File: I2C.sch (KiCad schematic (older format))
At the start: 10 parts

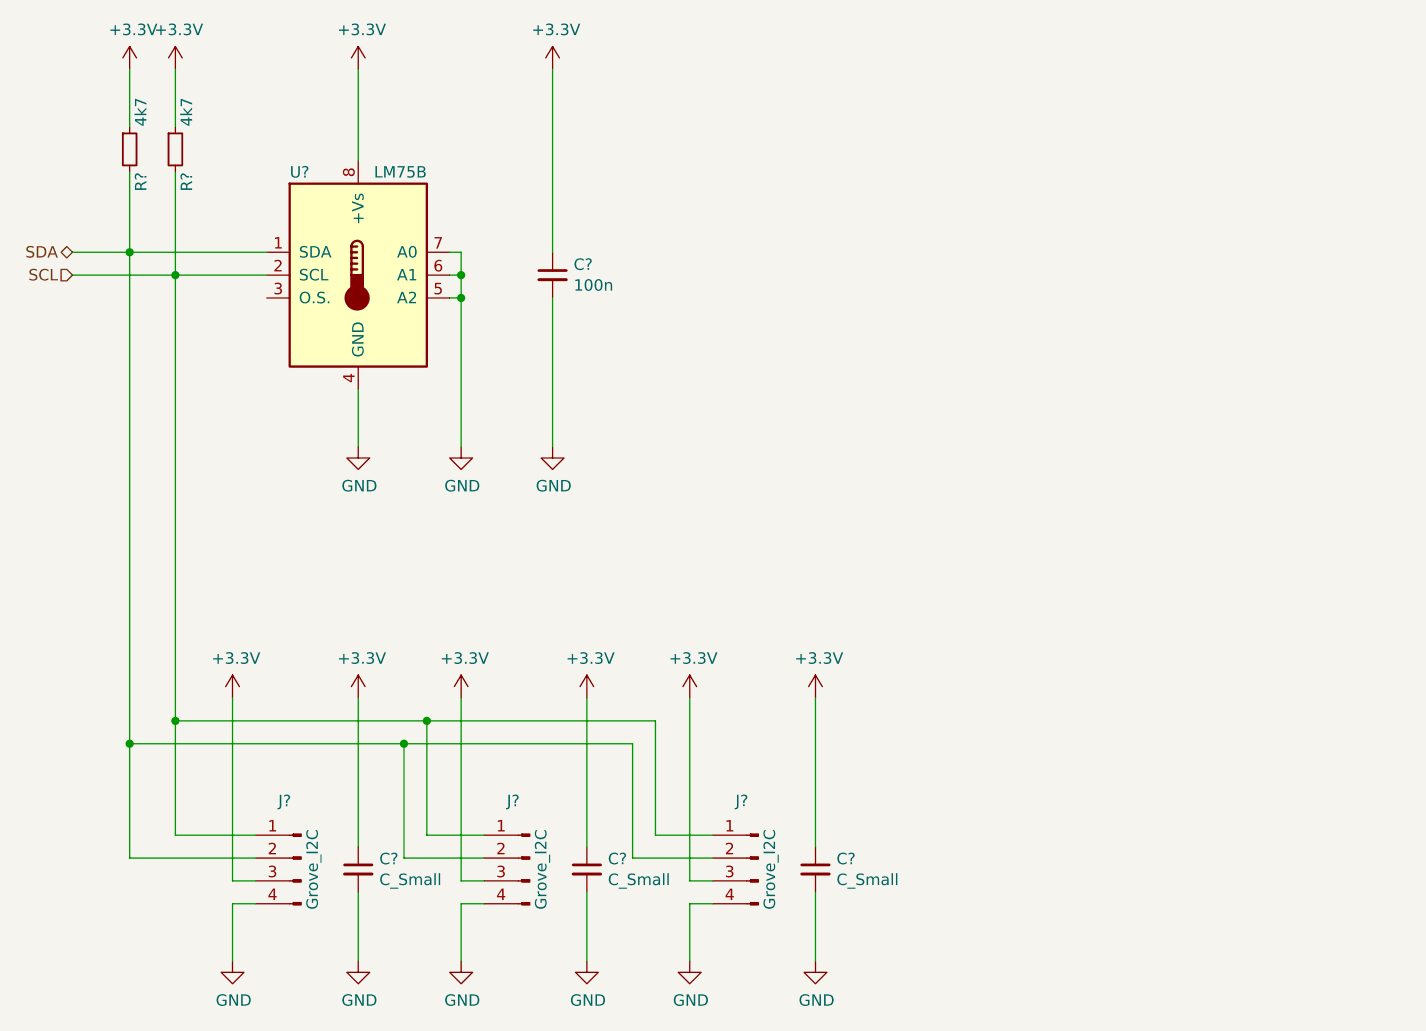
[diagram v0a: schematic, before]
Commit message: Erste fertige Version
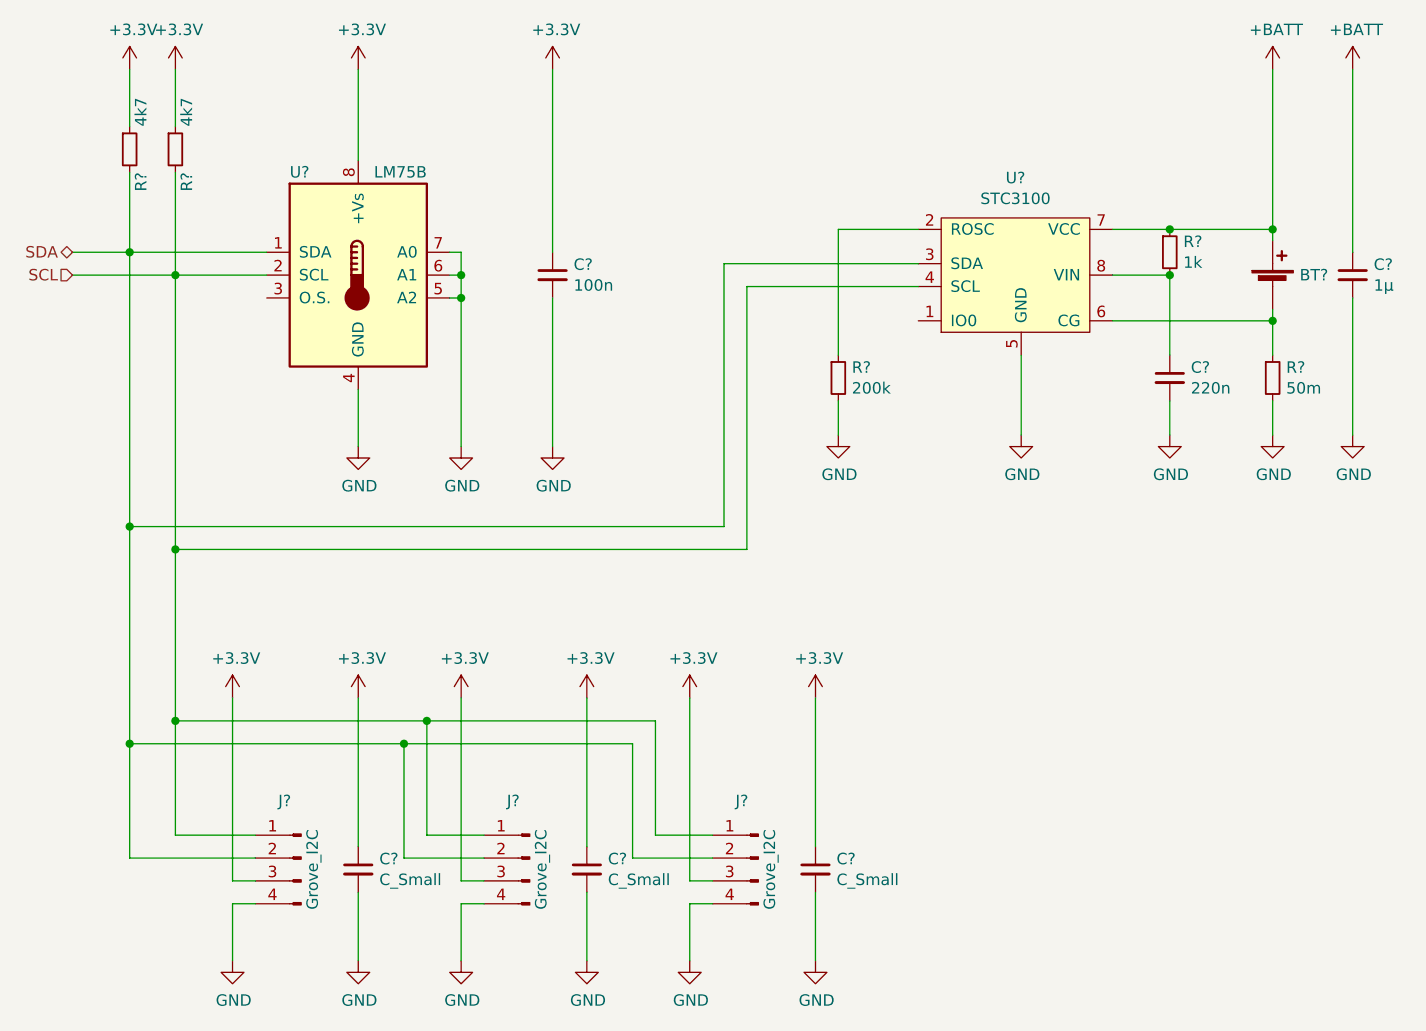
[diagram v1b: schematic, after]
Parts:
- added BT?: Battery_Cell, symbol Device:Battery_Cell
- added C?: 220n, symbol Device:C_Small
- added C?: 1µ, symbol Device:C_Small
- added R?: 200k, symbol Device:R_Small
- added R?: 50m, symbol Device:R_Small
- added R?: 1k, symbol Device:R_Small
- added U?: STC3100, symbol HS-Wismar:STC3100
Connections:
- net GND: now also C?.2, C?.2, R?.2, R?.2, U?.5 (GND)
- net SCL: now also U?.4 (SCL)
- net SDA: now also U?.3 (SDA)
- new net: R?.1, U?.2 (ROSC)
- new net: BT?.2 (-), R?.1, U?.6 (CG)
- new net: C?.1, R?.2, U?.8 (VIN)
- new net +BATT: BT?.1 (+), C?.1, R?.1, U?.7 (VCC)
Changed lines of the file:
@@
 $Descr A4 11693 8268
 encoding utf-8
-Sheet 9 10
+Sheet 8 10
 Title ""
 Date ""
@@
 $EndComp
 Wire Wire Line
-	2450 2250 2450 4400
-Wire Wire Line
-	2650 4300 2650 2350
+	2450 2250 2450 3450
+Wire Wire Line
+	2650 4300 2650 3550
 $Comp
 L power:GND #PWR?
@@
 Wire Wire Line
 	5450 5350 5450 5050
+$Comp
+L HS-Wismar:STC3100 U?
+U 1 1 5F025B7B
+P 6000 2600
+F 0 "U?" H 6325 3275 50  0000 C CNN
+F 1 "STC3100" H 6325 3184 50  0000 C CNN
+F 2 "" H 6000 2600 50  0001 C CNN
+F 3 "" H 6000 2600 50  0001 C CNN
+	1    6000 2600
+	1    0    0    -1
+$EndComp
+Wire Wire Line
+	5900 2300 5050 2300
+Wire Wire Line
+	5050 2300 5050 3450
+Wire Wire Line
+	5050 3450 2450 3450
+Connection ~ 2450 3450
+Wire Wire Line
+	2450 3450 2450 4400
+Wire Wire Line
+	5900 2400 5150 2400
+Wire Wire Line
+	5150 2400 5150 3550
+Wire Wire Line
+	5150 3550 2650 3550
+Connection ~ 2650 3550
+Wire Wire Line
+	2650 3550 2650 2350
+$Comp
+L Device:R_Small R?
+U 1 1 5F02B055
+P 5550 2800
+F 0 "R?" H 5609 2846 50  0000 L CNN
+F 1 "200k" H 5609 2755 50  0000 L CNN
+F 2 "" H 5550 2800 50  0001 C CNN
+F 3 "~" H 5550 2800 50  0001 C CNN
+	1    5550 2800
+	1    0    0    -1
+$EndComp
+Wire Wire Line
+	5550 2700 5550 2150
+Wire Wire Line
+	5550 2150 5900 2150
+$Comp
+L power:GND #PWR?
+U 1 1 5F02CA9E
+P 5550 3050
+F 0 "#PWR?" H 5550 2800 50  0001 C CNN
+F 1 "GND" H 5555 2877 50  0000 C CNN
+F 2 "" H 5550 3050 50  0001 C CNN
+F 3 "" H 5550 3050 50  0001 C CNN
+	1    5550 3050
+	1    0    0    -1
+$EndComp
+Wire Wire Line
+	5550 3050 5550 2900
+$Comp
+L Device:Battery_Cell BT?
+U 1 1 5F02E8A9
+P 7450 2400
+F 0 "BT?" H 7568 2450 50  0000 L CNN
+F 1 "Battery_Cell" H 7568 2405 50  0001 L CNN
+F 2 "" V 7450 2460 50  0001 C CNN
+F 3 "~" V 7450 2460 50  0001 C CNN
+	1    7450 2400
+	1    0    0    -1
+$EndComp
+$Comp
+L Device:R_Small R?
+U 1 1 5F031F1C
+P 7450 2800
+F 0 "R?" H 7509 2846 50  0000 L CNN
+F 1 "50m" H 7509 2755 50  0000 L CNN
+F 2 "" H 7450 2800 50  0001 C CNN
+F 3 "~" H 7450 2800 50  0001 C CNN
+	1    7450 2800
+	1    0    0    -1
+$EndComp
+Wire Wire Line
+	6750 2550 7450 2550
+Wire Wire Line
+	7450 2550 7450 2500
+Wire Wire Line
+	7450 2550 7450 2700
+Connection ~ 7450 2550
+$Comp
+L power:GND #PWR?
+U 1 1 5F035075
+P 7450 3050
+F 0 "#PWR?" H 7450 2800 50  0001 C CNN
+F 1 "GND" H 7455 2877 50  0000 C CNN
+F 2 "" H 7450 3050 50  0001 C CNN
+F 3 "" H 7450 3050 50  0001 C CNN
+	1    7450 3050
+	1    0    0    -1
+$EndComp
+Wire Wire Line
+	7450 3050 7450 2900
+Wire Wire Line
+	6750 2150 7000 2150
+Wire Wire Line
+	7450 2150 7450 2200
+$Comp
+L power:+BATT #PWR?
+U 1 1 5F038F3C
+P 7450 1450
+F 0 "#PWR?" H 7450 1300 50  0001 C CNN
+F 1 "+BATT" H 7465 1623 50  0000 C CNN
+F 2 "" H 7450 1450 50  0001 C CNN
+F 3 "" H 7450 1450 50  0001 C CNN
+	1    7450 1450
+	1    0    0    -1
+$EndComp
+Wire Wire Line
+	7450 1450 7450 2150
+Connection ~ 7450 2150
+$Comp
+L Device:C_Small C?
+U 1 1 5F03D903
+P 7000 2800
+F 0 "C?" H 7092 2846 50  0000 L CNN
+F 1 "220n" H 7092 2755 50  0000 L CNN
+F 2 "" H 7000 2800 50  0001 C CNN
+F 3 "~" H 7000 2800 50  0001 C CNN
+	1    7000 2800
+	1    0    0    -1
+$EndComp
+$Comp
+L Device:C_Small C?
+U 1 1 5F03E815
+P 7800 2350
+F 0 "C?" H 7892 2396 50  0000 L CNN
+F 1 "1µ" H 7892 2305 50  0000 L CNN
+F 2 "" H 7800 2350 50  0001 C CNN
+F 3 "~" H 7800 2350 50  0001 C CNN
+	1    7800 2350
+	1    0    0    -1
+$EndComp
+$Comp
+L Device:R_Small R?
+U 1 1 5F03EB5A
+P 7000 2250
+F 0 "R?" H 7059 2296 50  0000 L CNN
+F 1 "1k" H 7059 2205 50  0000 L CNN
+F 2 "" H 7000 2250 50  0001 C CNN
+F 3 "~" H 7000 2250 50  0001 C CNN
+	1    7000 2250
+	1    0    0    -1
+$EndComp
+Connection ~ 7000 2150
+Wire Wire Line
+	7000 2150 7450 2150
+Wire Wire Line
+	6750 2350 7000 2350
+Wire Wire Line
+	7000 2350 7000 2700
+Connection ~ 7000 2350
+$Comp
+L power:GND #PWR?
+U 1 1 5F041DCD
+P 7000 3050
+F 0 "#PWR?" H 7000 2800 50  0001 C CNN
+F 1 "GND" H 7005 2877 50  0000 C CNN
+F 2 "" H 7000 3050 50  0001 C CNN
+F 3 "" H 7000 3050 50  0001 C CNN
+	1    7000 3050
+	1    0    0    -1
+$EndComp
+Wire Wire Line
+	7000 3050 7000 2900
+$Comp
+L power:+BATT #PWR?
+U 1 1 5F044900
+P 7800 1450
+F 0 "#PWR?" H 7800 1300 50  0001 C CNN
+F 1 "+BATT" H 7815 1623 50  0000 C CNN
+F 2 "" H 7800 1450 50  0001 C CNN
+F 3 "" H 7800 1450 50  0001 C CNN
+	1    7800 1450
+	1    0    0    -1
+$EndComp
+Wire Wire Line
+	7800 1450 7800 2250
+$Comp
+L power:GND #PWR?
+U 1 1 5F0476E8
+P 7800 3050
+F 0 "#PWR?" H 7800 2800 50  0001 C CNN
+F 1 "GND" H 7805 2877 50  0000 C CNN
+F 2 "" H 7800 3050 50  0001 C CNN
+F 3 "" H 7800 3050 50  0001 C CNN
+	1    7800 3050
+	1    0    0    -1
+$EndComp
+Wire Wire Line
+	7800 3050 7800 2450
+$Comp
+L power:GND #PWR?
+U 1 1 5F04B71B
+P 6350 3050
+F 0 "#PWR?" H 6350 2800 50  0001 C CNN
+F 1 "GND" H 6355 2877 50  0000 C CNN
+F 2 "" H 6350 3050 50  0001 C CNN
+F 3 "" H 6350 3050 50  0001 C CNN
+	1    6350 3050
+	1    0    0    -1
+$EndComp
+Wire Wire Line
+	6350 3050 6350 2700
 $EndSCHEMATC

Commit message: Externe Spannungsversorgung
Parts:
- BT?: value Battery_Cell -> 18650_Cell
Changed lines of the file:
@@
 P 7450 2400
 F 0 "BT?" H 7568 2450 50  0000 L CNN
-F 1 "Battery_Cell" H 7568 2405 50  0001 L CNN
+F 1 "18650_Cell" H 7568 2405 50  0001 L CNN
 F 2 "" V 7450 2460 50  0001 C CNN
 F 3 "~" V 7450 2460 50  0001 C CNN
